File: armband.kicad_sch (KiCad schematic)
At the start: 14 parts, among them IC1 QSMP-1570, SW1 SW_MEC_5G, SW2 SW_MEC_5G

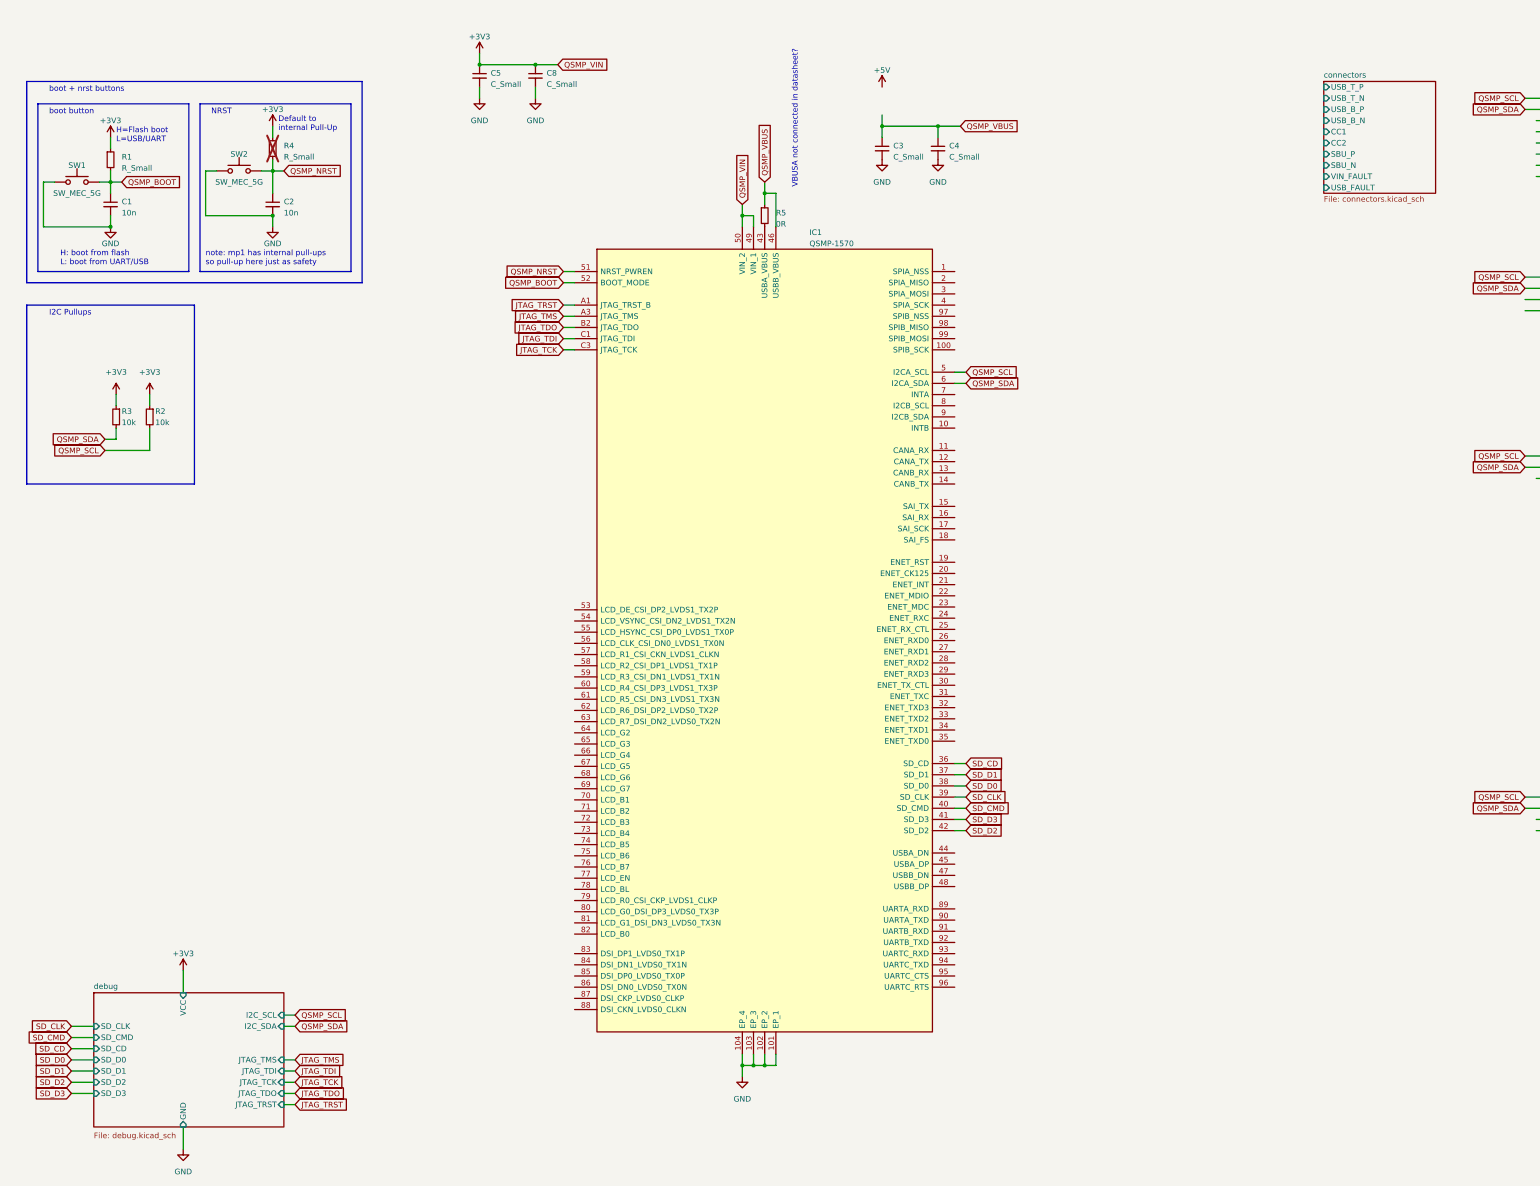
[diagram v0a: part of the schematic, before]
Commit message: finished usb connection ciruits
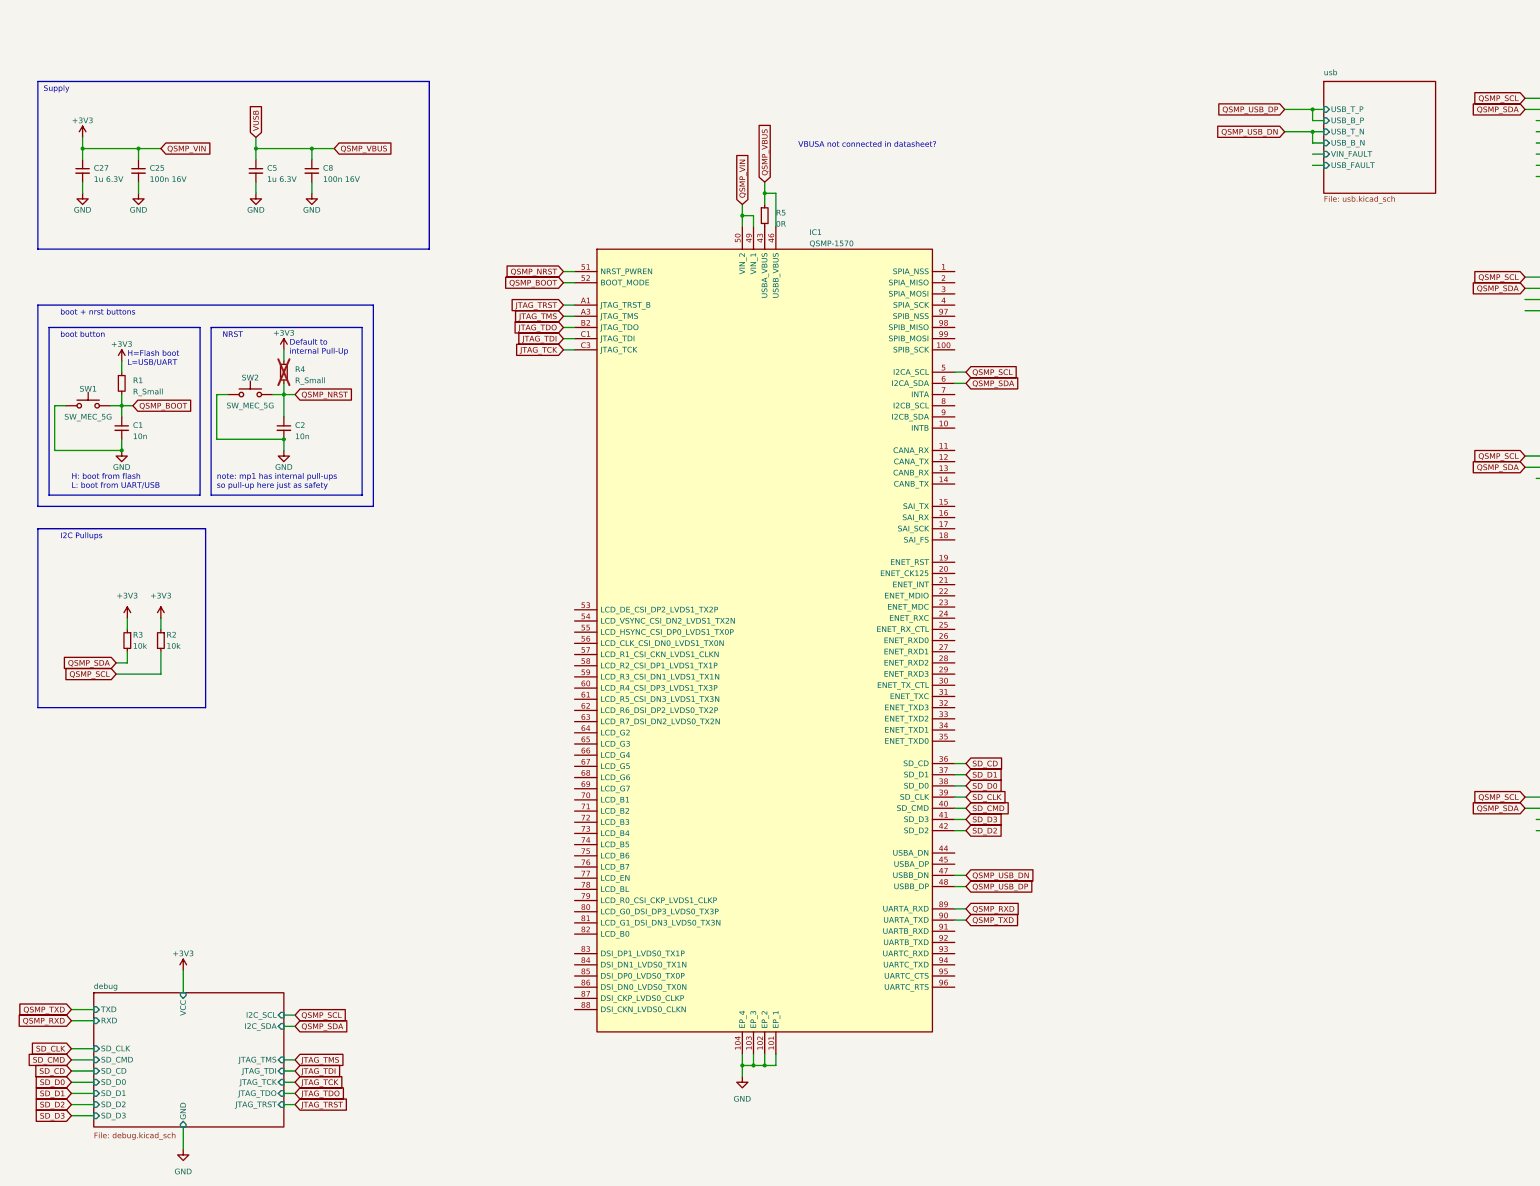
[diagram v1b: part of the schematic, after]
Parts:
- removed C3, C4: C_Small, symbol Device:C_Small
- added C25: 100n 16V, Capacitor_SMD:C_0402_1005Metric, symbol Device:C_Small
- added C27: 1u 6.3V, Capacitor_SMD:C_0201_0603Metric, symbol Device:C_Small
- C5: value C_Small -> 1u 6.3V; footprint (none) -> Capacitor_SMD:C_0201_0603Metric; MFN (none) -> 710-885012104011
- C8: value C_Small -> 100n 16V; footprint (none) -> Capacitor_SMD:C_0402_1005Metric; MFN (none) -> 80-C0402C104M4V
- R5: footprint Resistor_SMD:R_0402_1005Metric -> Resistor_SMD:R_0201_0603Metric; MFN (none) -> 603-AC0201JR-070RL
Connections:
- net +3V3: now also C25.1, C27.1; no longer C5.1, C8.1
- net GND: now also C25.2, C27.2
- net QSMP_VBUS: now also C5.1, C8.1
- net QSMP_USB_DN: now reaches IC1.47 (USBB_DN)
- net QSMP_USB_DP: now reaches IC1.48 (USBB_DP)
- net QSMP_RXD: now reaches IC1.89 (UARTA_RXD)
- net QSMP_TXD: now reaches IC1.90 (UARTA_TXD)
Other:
- sheet connectors renamed usb
- sheet debug ports: added RXD, TXD; removed none
- sheet usb: file connectors.kicad_sch -> usb.kicad_sch
- sheet usb ports: added none; removed CC1, CC2, SBU_N, SBU_P
- note added: "Supply"
- moved on the sheet: C1, C2, R1, R2, R3, R4, SW1, SW2
